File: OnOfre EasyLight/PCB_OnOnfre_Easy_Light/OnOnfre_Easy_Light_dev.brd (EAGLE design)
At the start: 44.5 x 45.5 mm, 27 parts, among them J3Y S8050, K1 OMRON-G3MB-202P-SSR2, K2 OMRON-G3MB-202P-SSR2, U2 esp12

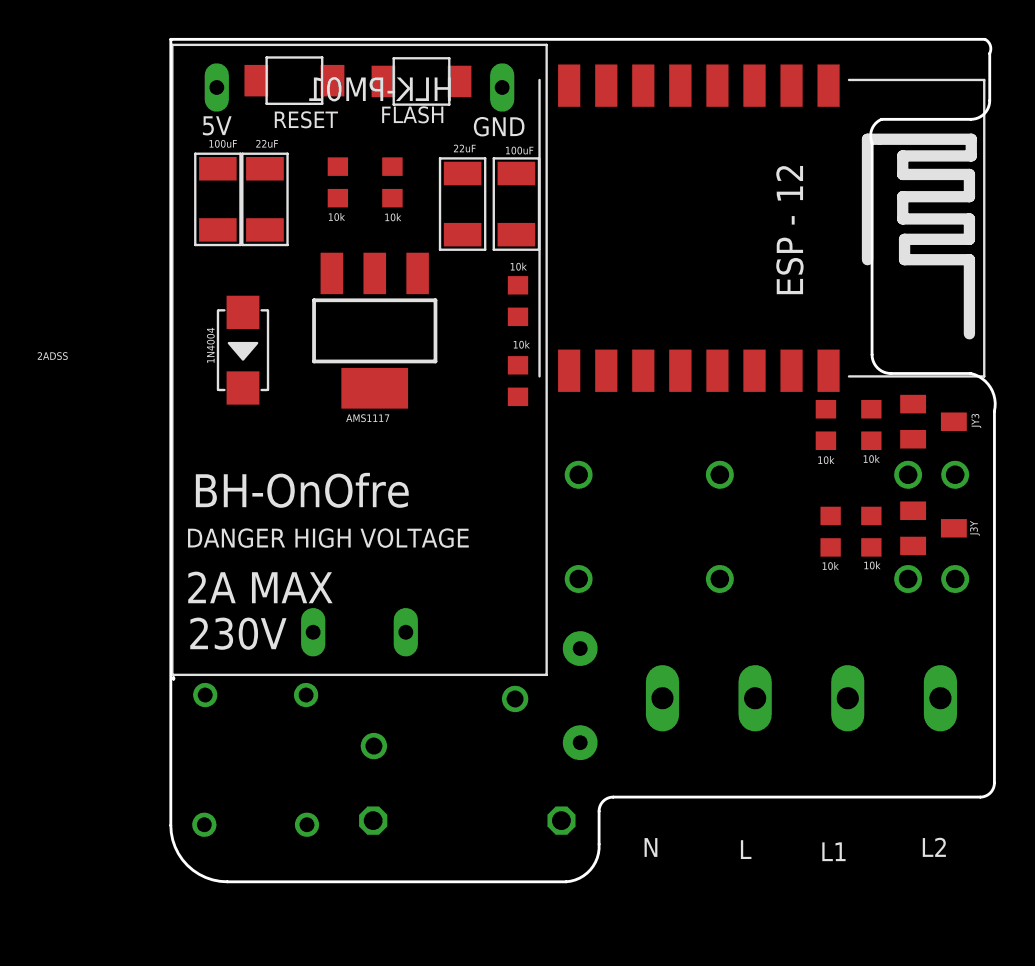
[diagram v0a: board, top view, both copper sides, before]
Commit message: no message
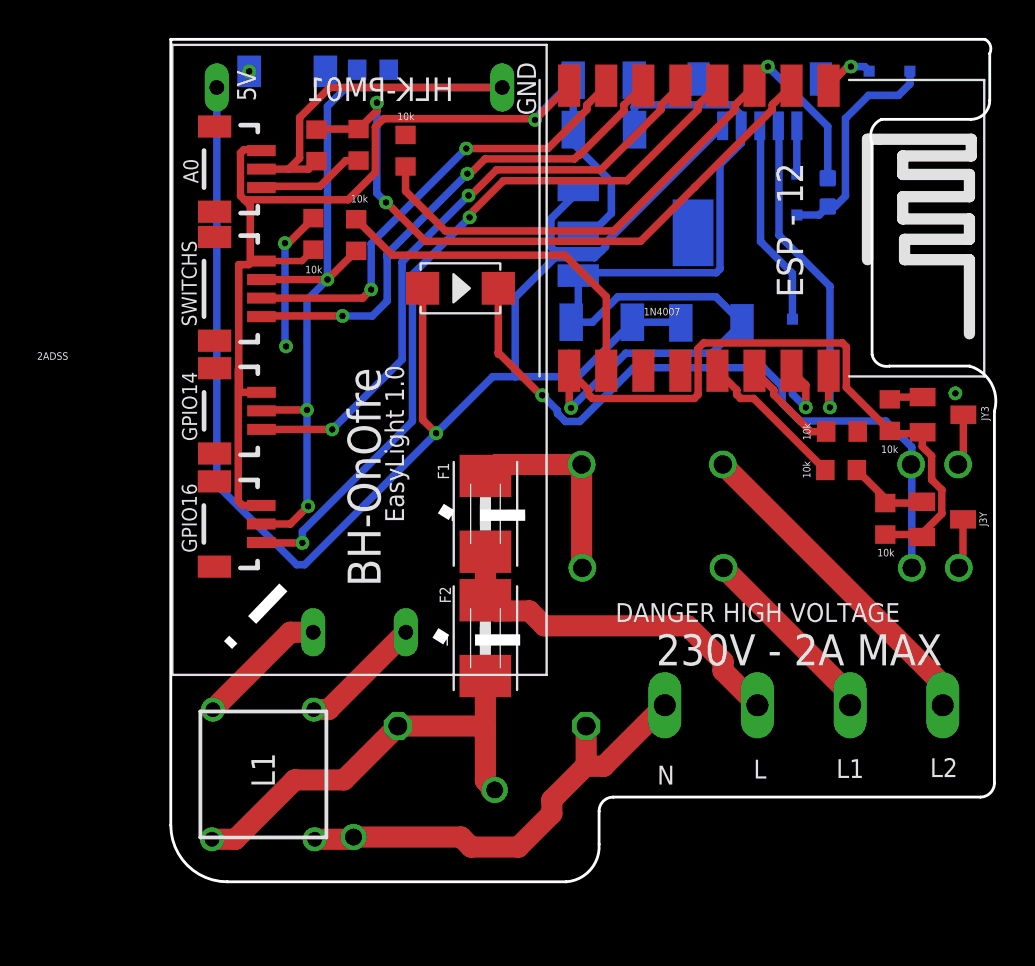
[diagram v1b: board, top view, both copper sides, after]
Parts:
- removed FLASH: B3U-1000P-2P-SMD, switches:B3U-1000P
- added A0, GPIO14, GPIO16: BM03B-SRSS-TB, con-jst2:BM03B-SRSS-TB
- added C6: 100nf, Seeed-Capacitor:C0603
- added D1, D2, D4: (no value), diode:SOD323-R
- added F2: (no value), adafruit:1812
- added FTDI: BM05B-SRSS-TB, con-jst2:BM05B-SRSS-TB
- added R6: 100k, resistor:R0603
- added R7: 220k, resistor:R0603
- added SWITCHS: BM04B-SRSS-TB, con-jst2:BM04B-SRSS-TB
- C1, C2: value 22uF -> 22uf
- C3, C4: value 100uF -> 100uf
- D3: value 1N4004 -> 1N4007
- F1: value 0.5A -> (none); device SparkFun-Fuses:PTH -> adafruit:1812
- moved C3 27.5 mm to (29.4, 31.2), flipped to the bottom, turned to 180 degrees
- moved C2 19.3 mm to (23.5, 31.2), flipped to the bottom, turned to 0 degrees
- moved AMS1117 15.0 mm to (25.3, 36.0), flipped to the bottom, turned to 90 degrees
- moved D3 12.2 mm to (15.9, 33.0), turned to 0 degrees
- moved R11 11.8 mm to (10.3, 35.9)
- moved F1 11.1 mm to (17.2, 20.9), flipped to the top
- moved R9 10.1 mm to (12.9, 40.5)
- moved C1 8.62 mm to (23.6, 41.6), flipped to the bottom, turned to 180 degrees
- moved C4 8.18 mm to (23.6, 44.3), flipped to the bottom, turned to 180 degrees
- moved R10 6.37 mm to (11.2, 44.8), flipped to the bottom, turned to 0 degrees
- moved C5 5.28 mm to (17.6, 9.42), turned to 180 degrees
- moved R8 5.09 mm to (7.95, 36.0)
- moved R5 5.03 mm to (13.9, 4.70)
- moved R4 3.37 mm to (36.4, 23.2), turned to 0 degrees
- moved R2 1.13 mm to (39.1, 26.2)
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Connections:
- removed net 3V3: AMS1117.2, C1.1, C4.1, R10.2, R8.2, R9.2, U2.VCC
- removed net VCC: AMS1117.3, C2.1, C3.1, D3.1, U$2.P$4
- new net A0: A0.3, R7.2
- new net DTR: D2.C, FTDI.5
- new net LIVE_FUSED: F1.2, K1.1, K2.1
- new net N$3: D1.C, FTDI.3
- new net N$4: C6.2, D2.A, D4.C
- new net VCC_1: AMS1117.3, C2.1, C3.1, D3.1, FTDI.1, U$2.P$4
- new net VCC_2: A0.1, AMS1117.2, C1.1, C4.1, GPIO14.1, GPIO16.1, R10.2, R8.2, R9.2, SWITCHS.1, U2.VCC
- net ADC: now also R6.2, R7.1
- net CH_PD: now also C6.1
- net GND: now also A0.2, FTDI.2, GPIO14.2, GPIO16.2, R6.1, SWITCHS.2; no longer FLASH.2
- net GPIO0: no longer FLASH.1
- net GPIO12: now also SWITCHS.4
- net GPIO13: now also SWITCHS.3
- net GPIO14: now also GPIO14.3
- net GPIO16: now also GPIO16.3
- net LIVE: now also F1.1, F2.1; no longer F1.P$1, K1.1, K2.1
- net N$2: now also F2.2; no longer F1.P$2
- net RESET: now also D4.A
- net RX: now also D1.A
- net TX: now also FTDI.4
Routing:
- net GND: track 0.00 -> 149.0 mm, vias 0 -> 5
- net VCC_1: track 0.00 -> 87.8 mm, vias 0 -> 1
- net VCC_2: track 0.00 -> 63.6 mm, vias 0 -> 1
- net GPIO16: track 0.00 -> 40.1 mm, vias 0 -> 2
- net 5V: track 0.00 -> 37.6 mm, vias 0 -> 1
- net ADC: track 0.00 -> 36.1 mm, vias 0 -> 2
- net GPIO14: track 0.00 -> 33.5 mm, vias 0 -> 2
- net CH_PD: track 0.00 -> 33.1 mm, vias 0 -> 1
- net GPIO12: track 0.00 -> 27.4 mm, vias 0 -> 2
- net NEUTRAL: track 0.00 -> 25.0 mm
- net GPIO13: track 0.00 -> 25.0 mm, vias 0 -> 2
- net N$2: track 0.00 -> 24.6 mm
- net LIVE: track 0.00 -> 20.0 mm
- net GPIO15: track 0.00 -> 19.2 mm
- net TX: track 0.00 -> 18.4 mm, vias 0 -> 1
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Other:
- outline, holes or cut-outs redrawn
- board text added: "230V - 2A MAX"
- board text added: "EasyLight 1.0"
- board text removed: "230V"
- board text removed: "2A MAX"
- board text removed: "HLK-PM01"

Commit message: versão beta 1
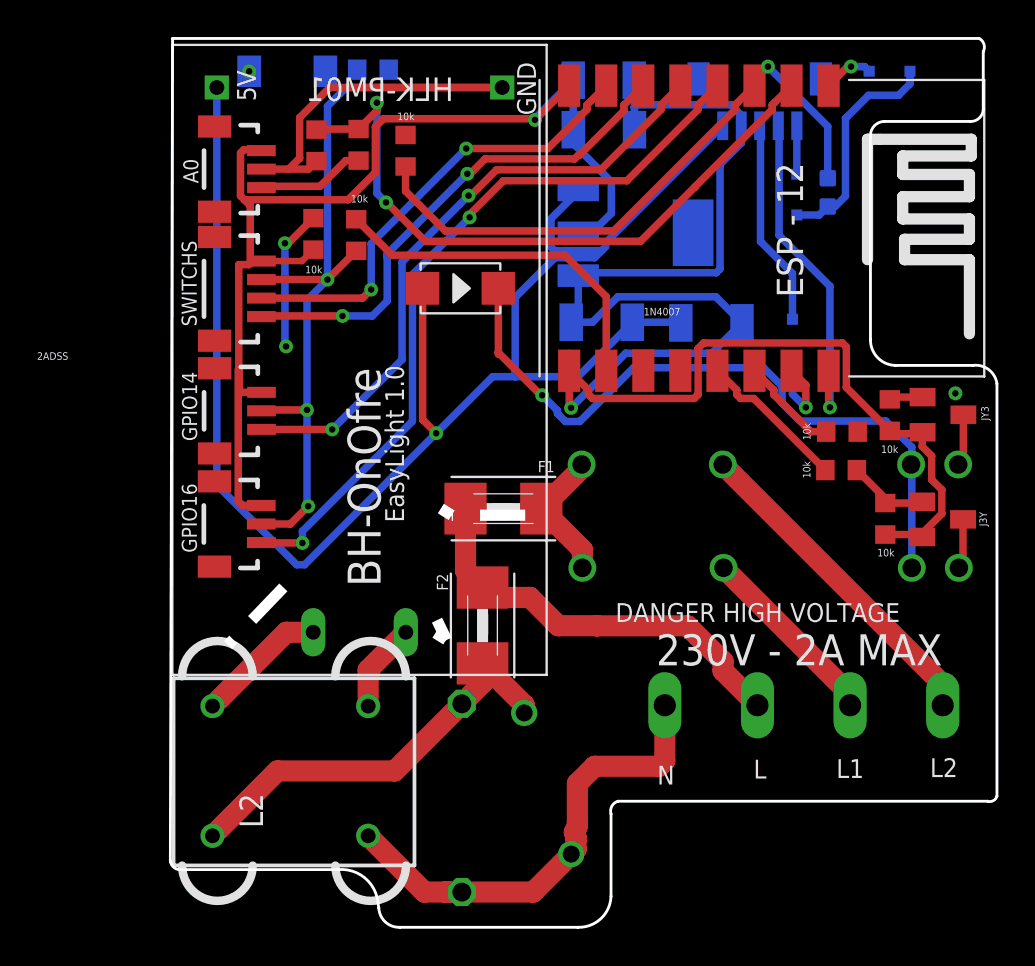
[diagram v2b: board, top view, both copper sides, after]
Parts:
- removed L1: (no value), inductor-neosid:ZD6-2X15
- added L2: (no value), inductor-onofre:ZD6-2X15
- moved R5 6.86 mm to (20.6, 6.32), turned to 0 degrees
- moved C5 4.21 mm to (16.0, 5.54), turned to 270 degrees
- moved F1 1.01 mm to (18.2, 21.2), turned to 0 degrees
- moved F2 0.70 mm to (17.1, 14.8)
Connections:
- net EMI_LIVE: now also L2.4; no longer L1.2
- net EMI_NEUTRAL: now also L2.3; no longer L1.1
- net N$2: now also L2.1; no longer L1.3
- net NEUTRAL: now also L2.2; no longer L1.4
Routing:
- net LIVE_FUSED: track 11.9 -> 7.40 mm
- net LIVE: track 20.0 -> 22.4 mm
- net EMI_NEUTRAL: track 6.69 -> 4.83 mm
- net N$2: track 24.6 -> 23.4 mm
- net NEUTRAL: track 25.0 -> 26.2 mm
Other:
- board size 44.5 x 45.5 mm -> 44.6 x 48 mm
